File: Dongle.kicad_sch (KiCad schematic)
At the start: 43 parts, among them J1 USB_A, J2 TC2050-IDC

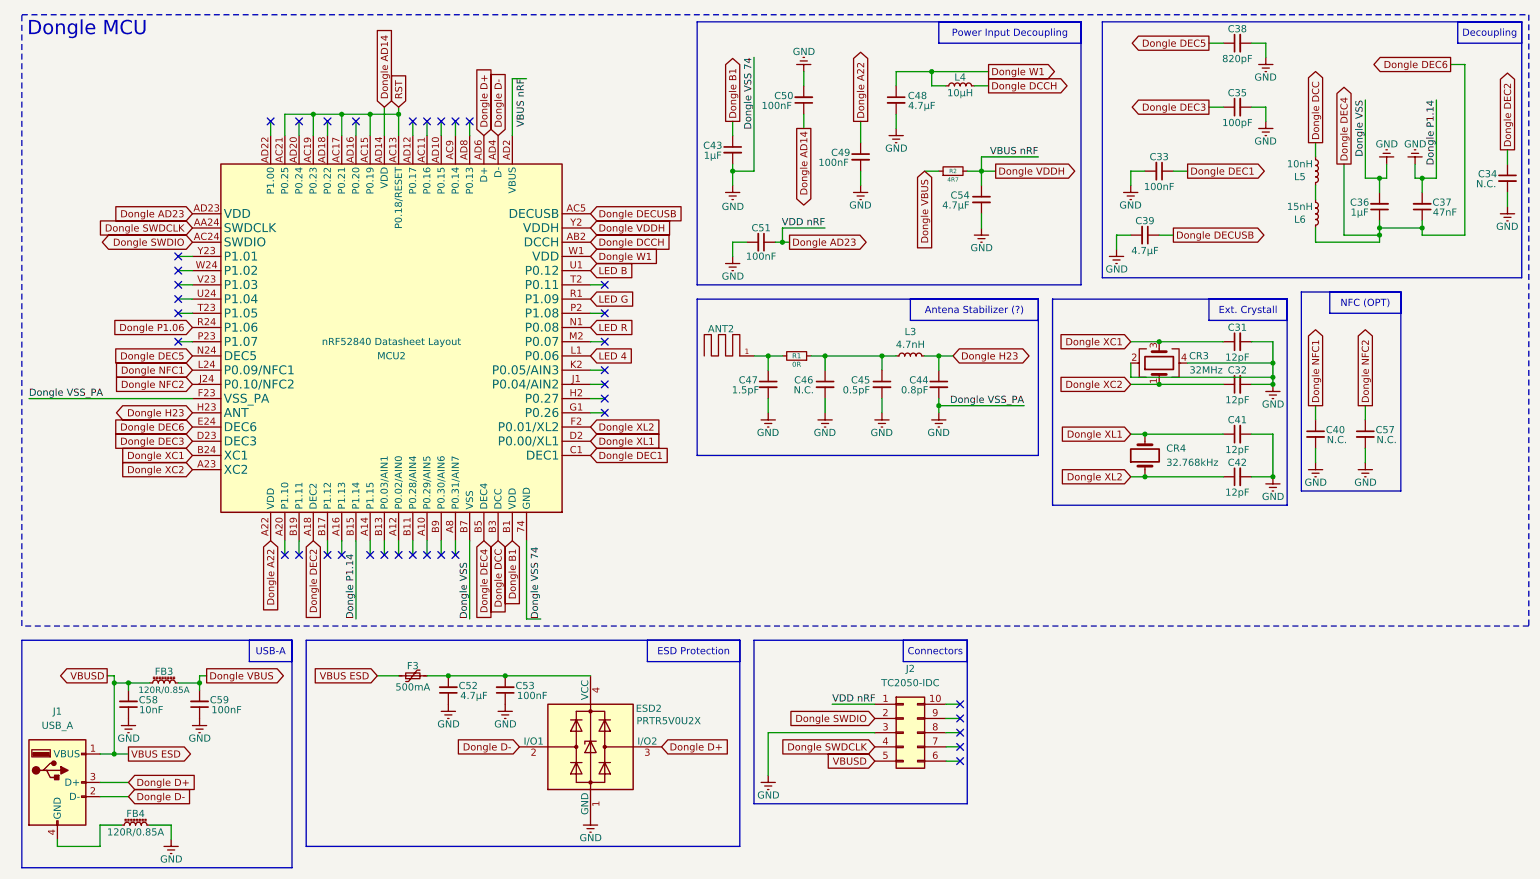
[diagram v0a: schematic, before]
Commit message: 8th commit
Some minor tweak
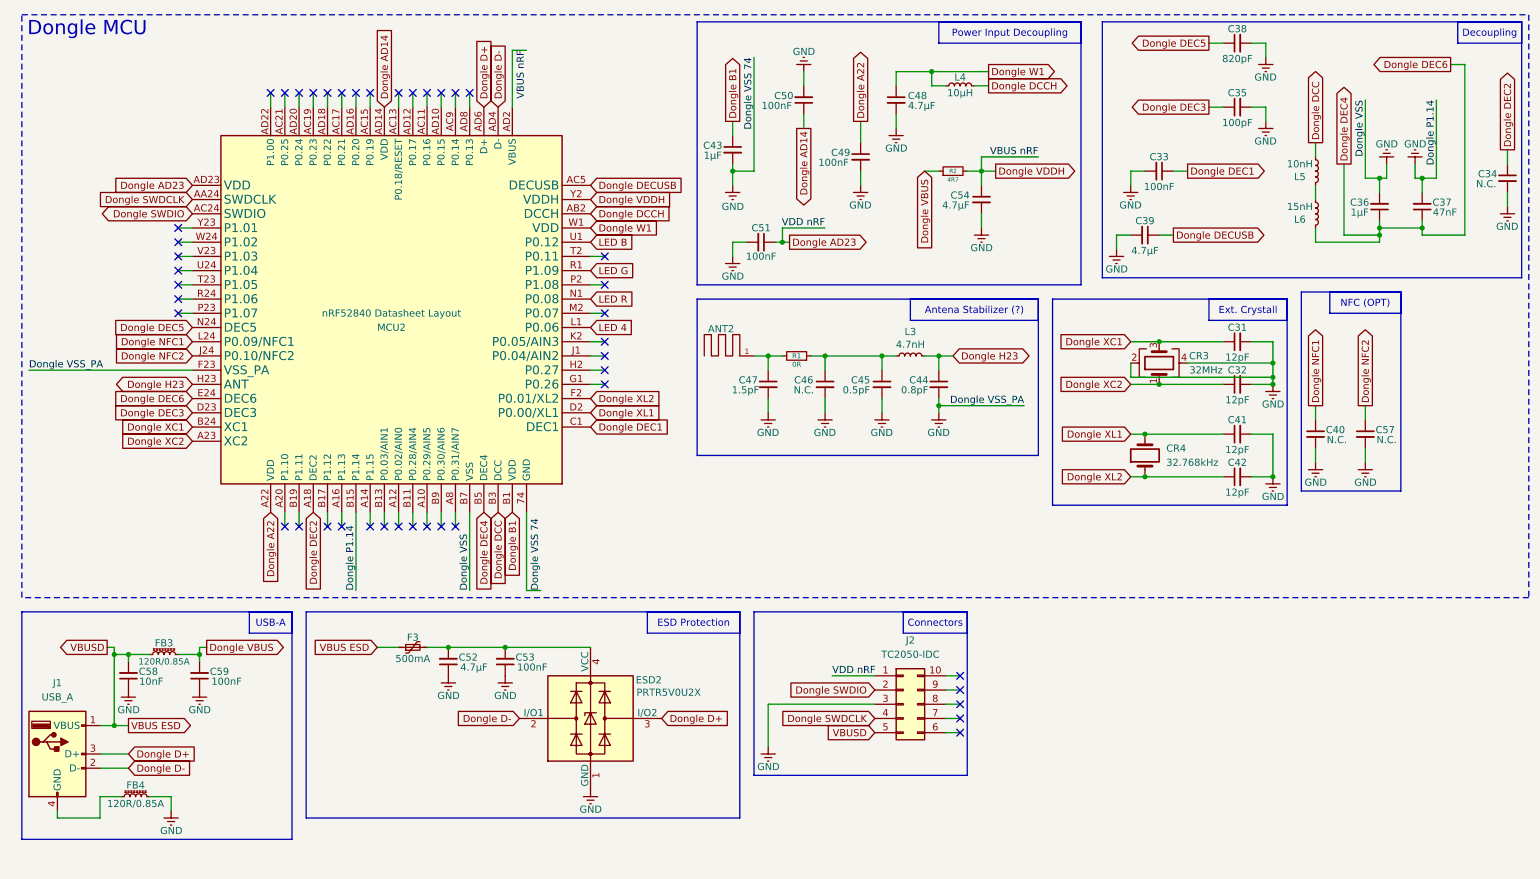
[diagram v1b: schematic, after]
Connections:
- net Dongle P1.06: no longer names the net of MCU2.R24 (P1.06)
- removed net RST: MCU2.AC13 (P0.18/RESET), MCU2.AC15 (P0.19), MCU2.AC17 (P0.21), MCU2.AC19 (P0.23), MCU2.AC21 (P0.25)
- no-connect marks 38 -> 44
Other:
- moved on the sheet: C52, C53, C58, C59, ESD2, F3, FB3, FB4, J1, J2, MCU2
